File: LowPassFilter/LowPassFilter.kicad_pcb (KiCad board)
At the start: 2 copper layers, 34.5 x 26.4 mm, 11 parts, among them J1 OUT, J2 INP, T1 DoubleWindingTransformer

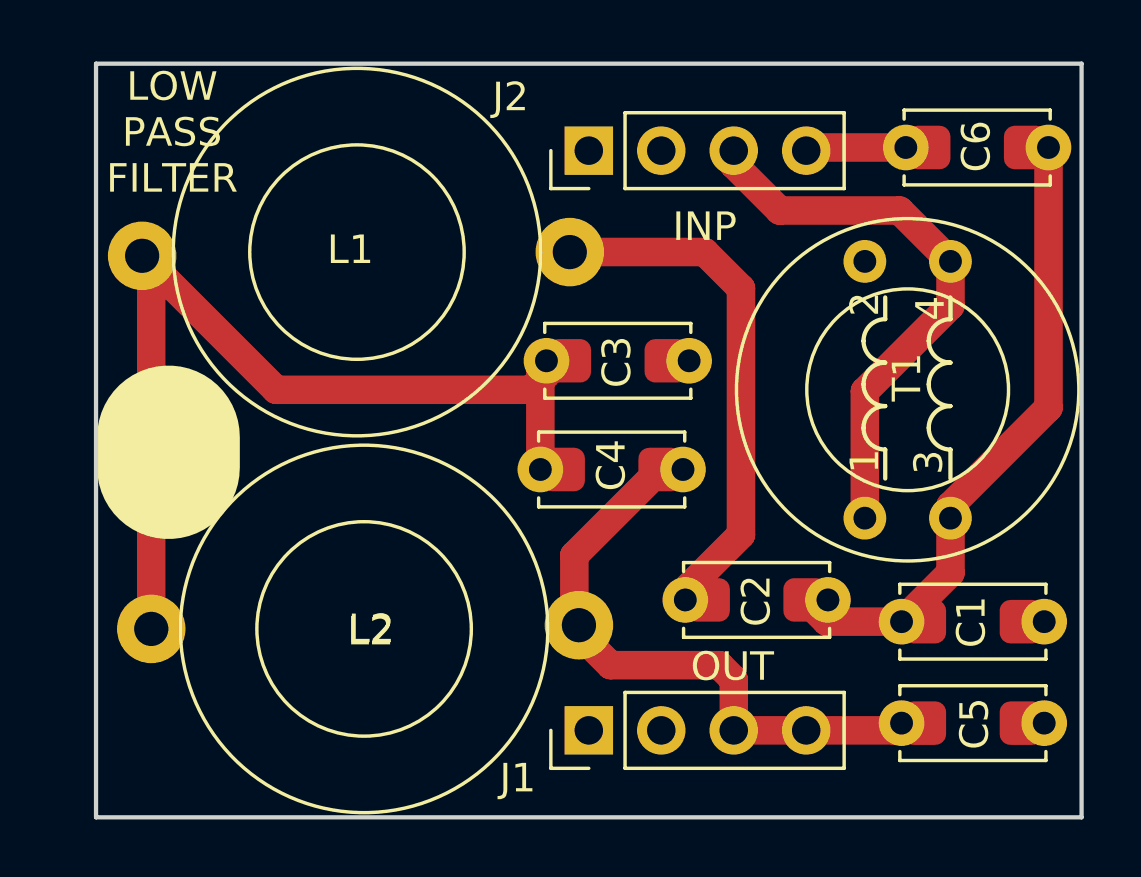
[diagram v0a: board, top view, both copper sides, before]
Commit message: JLCPCB order
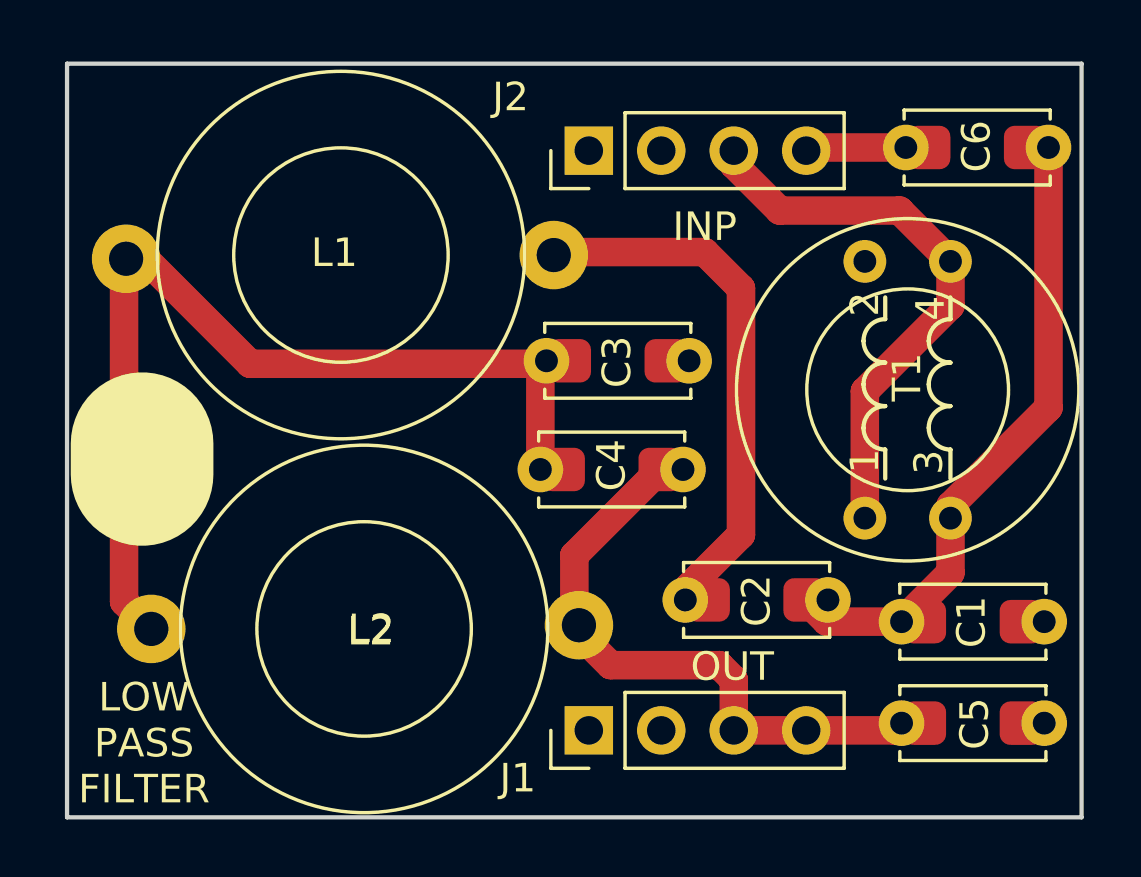
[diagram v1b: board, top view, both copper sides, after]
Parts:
- moved L1 0.57 mm to (133.9, 95.1)
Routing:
- net Net-(C2-Pad2): track 18.3 -> 18.9 mm
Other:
- board size 34.5 x 26.4 mm -> 35.6 x 26.4 mm
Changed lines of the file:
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@@
   )
   (footprint "LowPassFilter:L_Toroid_Horizontal_D12.7mm_Compact" (layer "F.Cu")
-    (at 134.462 94.996 180)
+    (at 133.9 95.1 180)
     (descr "L_Toroid, Horizontal series, Radial, pin pitch=20.00mm, , diameter=12.7mm,Compact")
     (tags "L_Toroid Horizontal series Radial pin pitch 20.00mm  diameter 12.7mm Diameter14-5mm Amidon-T50")
@@
     )
   )
-  (gr_line (start 117.856 102.5525) (end 117.856 101.473) (layer "F.SilkS") (width 5))
-  (gr_line (start 115.316 88.392) (end 149.86 88.392) (layer "Edge.Cuts") (width 0.15))
-  (gr_line (start 149.86 114.808) (end 115.316 114.808) (layer "Edge.Cuts") (width 0.15))
-  (gr_line (start 115.316 114.808) (end 115.316 88.392) (layer "Edge.Cuts") (width 0.15))
+  (gr_line (start 116.93 102.79) (end 116.93 101.7105) (layer "F.SilkS") (width 5))
+  (gr_line (start 114.3 88.392) (end 149.86 88.392) (layer "Edge.Cuts") (width 0.15))
+  (gr_line (start 149.86 114.808) (end 114.3 114.808) (layer "Edge.Cuts") (width 0.15))
+  (gr_line (start 114.3 114.808) (end 114.3 88.392) (layer "Edge.Cuts") (width 0.15))
   (gr_line (start 149.86 88.392) (end 149.86 114.808) (layer "Edge.Cuts") (width 0.15))
-  (gr_text "LOW\nPASS\nFILTER" (at 117.983 90.805) (layer "F.SilkS")
+  (gr_text "LOW\nPASS\nFILTER" (at 117 112.21) (layer "F.SilkS")
     (effects (font (size 1 1) (thickness 0.15)))
   )
@@
   (segment (start 145.264 103.886) (end 145.264 104.322) (width 1) (layer "F.Cu") (net 4))
   (segment (start 137.922 104.902) (end 135.97 106.854) (width 1) (layer "F.Cu") (net 5))
+  (segment (start 131.36 95.1) (end 131.464 94.996) (width 1) (layer "F.Cu") (net 5))
   (segment (start 136.652 94.996) (end 137.922 96.266) (width 1) (layer "F.Cu") (net 5))
-  (segment (start 131.922 94.996) (end 136.652 94.996) (width 1) (layer "F.Cu") (net 5))
+  (segment (start 131.464 94.996) (end 136.652 94.996) (width 1) (layer "F.Cu") (net 5))
+  (segment (start 137.922 96.266) (end 137.922 104.902) (width 1) (layer "F.Cu") (net 5))
   (segment (start 135.97 106.854) (end 135.97 107.188) (width 1) (layer "F.Cu") (net 5))
-  (segment (start 137.922 96.266) (end 137.922 104.902) (width 1) (layer "F.Cu") (net 5))
+  (segment (start 120.716 98.91) (end 131 98.91) (width 1) (layer "F.Cu") (net 6))
   (segment (start 130.89 102.616) (end 130.89 99.02) (width 1) (layer "F.Cu") (net 6))
-  (segment (start 117.252 95.446) (end 116.932 95.126) (width 1) (layer "F.Cu") (net 6))
-  (segment (start 121.628 99.822) (end 130.556 99.822) (width 1) (layer "F.Cu") (net 6))
-  (segment (start 131.104 99.274) (end 131.104 98.806) (width 1) (layer "F.Cu") (net 6))
-  (segment (start 130.556 99.822) (end 131.104 99.274) (width 1) (layer "F.Cu") (net 6))
-  (segment (start 116.932 95.126) (end 121.628 99.822) (width 1) (layer "F.Cu") (net 6))
+  (segment (start 117.252 108.204) (end 116.3 107.252) (width 1) (layer "F.Cu") (net 6))
+  (segment (start 116.3 95.3) (end 116.37 95.23) (width 1) (layer "F.Cu") (net 6))
+  (segment (start 116.37 95.23) (end 117.036 95.23) (width 1) (layer "F.Cu") (net 6))
+  (segment (start 131 98.91) (end 131.104 98.806) (width 1) (layer "F.Cu") (net 6))
   (segment (start 130.89 99.02) (end 131.104 98.806) (width 1) (layer "F.Cu") (net 6))
-  (segment (start 117.252 108.204) (end 117.252 95.446) (width 1) (layer "F.Cu") (net 6))
+  (segment (start 116.3 107.252) (end 116.3 95.3) (width 1) (layer "F.Cu") (net 6))
+  (segment (start 117.036 95.23) (end 120.716 98.91) (width 1) (layer "F.Cu") (net 6))
   (segment (start 137.16 109.474) (end 137.668 109.982) (width 1) (layer "F.Cu") (net 7))
   (segment (start 137.668 109.982) (end 137.668 111.76) (width 1) (layer "F.Cu") (net 7))
@@
       (pts
         (xy 149.86 114.808)
-        (xy 115.316 114.808)
-        (xy 115.316 88.392)
+        (xy 114.3 114.808)
+        (xy 114.3 88.392)
         (xy 149.86 88.392)
       )
